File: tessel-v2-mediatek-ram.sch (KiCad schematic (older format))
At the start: 21 parts, among them U201 MT7620N, U501 W9751G6KB-25

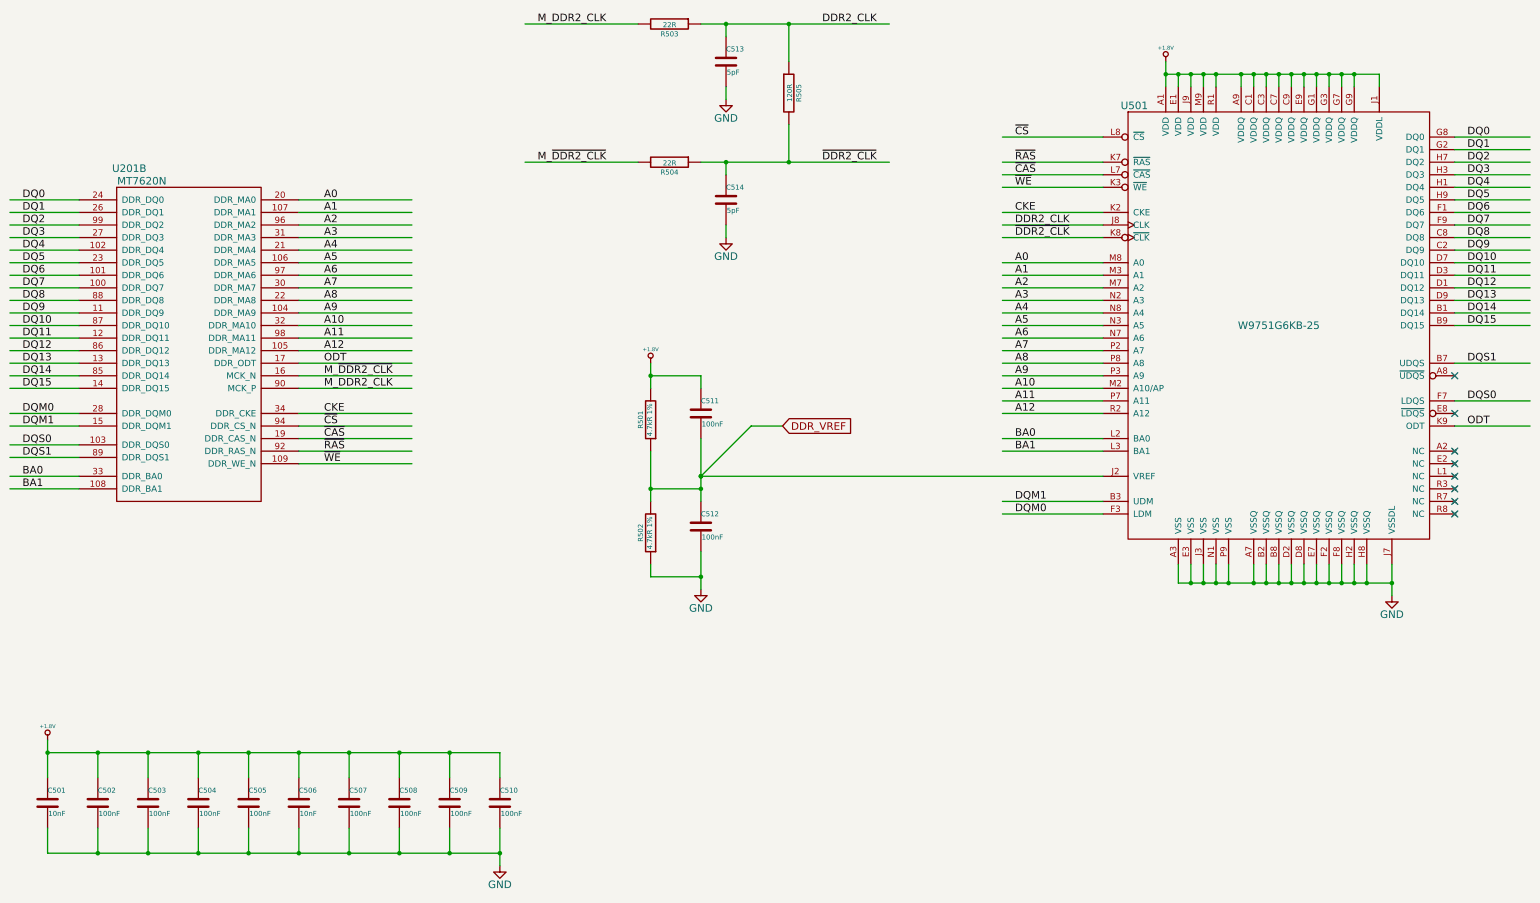
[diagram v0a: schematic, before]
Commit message: annotation did not take?
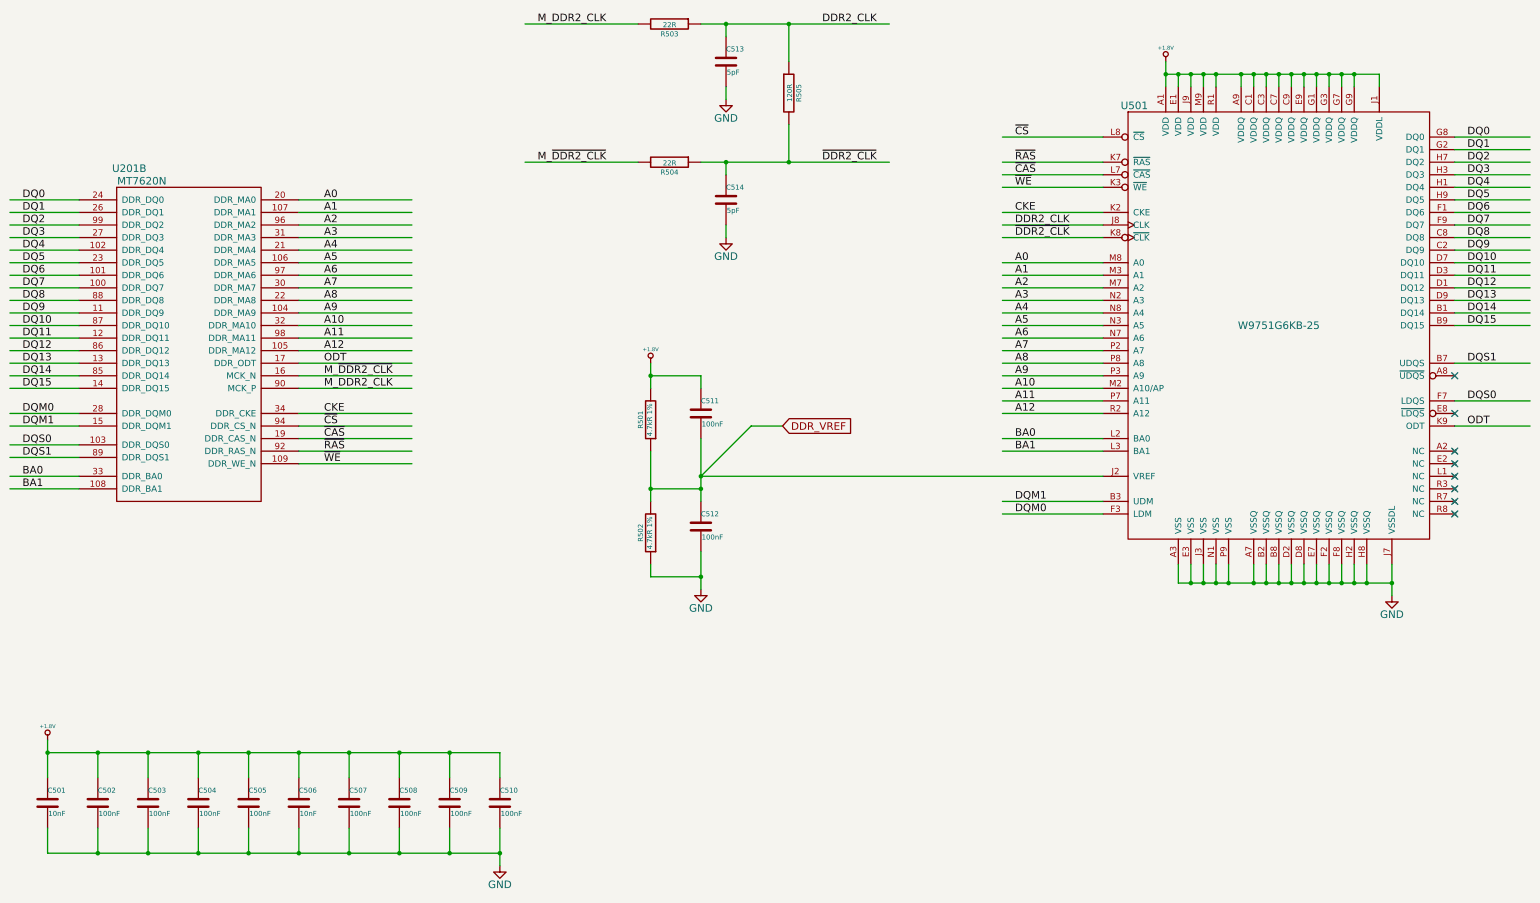
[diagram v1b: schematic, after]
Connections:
- wire segments 222 -> 164
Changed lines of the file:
@@
 	11500 7000 11500 7150
 Wire Wire Line
-	11500 7150 11600 7150
-Wire Wire Line
-	11600 7150 11700 7150
-Wire Wire Line
-	11700 7150 11800 7150
-Wire Wire Line
-	11800 7150 11900 7150
-Wire Wire Line
-	11900 7150 12100 7150
-Wire Wire Line
-	12100 7150 12200 7150
-Wire Wire Line
-	12200 7150 12300 7150
-Wire Wire Line
-	12300 7150 12400 7150
-Wire Wire Line
-	12400 7150 12500 7150
-Wire Wire Line
-	12500 7150 12600 7150
-Wire Wire Line
-	12600 7150 12700 7150
-Wire Wire Line
-	12700 7150 12800 7150
-Wire Wire Line
-	12800 7150 12900 7150
-Wire Wire Line
-	12900 7150 13000 7150
-Wire Wire Line
-	13000 7150 13200 7150
+	11500 7150 13200 7150
 Wire Wire Line
 	11600 7150 11600 7000
@@
 Connection ~ 12200 7150
 Wire Wire Line
-	13200 7000 13200 7150
-Wire Wire Line
-	13200 7150 13200 7250
+	13200 7000 13200 7250
 Wire Wire Line
 	12400 7150 12400 7000
@@
 	4500 5600 5400 5600
 Wire Wire Line
-	7700 2700 7900 2700
-Wire Wire Line
-	7900 2700 8400 2700
-Wire Wire Line
-	8400 2700 9200 2700
+	7700 2700 9200 2700
 Wire Wire Line
 	7900 2800 7900 2700
@@
 	6300 3800 7200 3800
 Wire Wire Line
-	11400 3100 11500 3100
-Wire Wire Line
-	11500 3100 11600 3100
-Wire Wire Line
-	11600 3100 11700 3100
-Wire Wire Line
-	11700 3100 11800 3100
-Wire Wire Line
-	11800 3100 12000 3100
-Wire Wire Line
-	12000 3100 12100 3100
-Wire Wire Line
-	12100 3100 12200 3100
-Wire Wire Line
-	12200 3100 12300 3100
-Wire Wire Line
-	12300 3100 12400 3100
-Wire Wire Line
-	12400 3100 12500 3100
-Wire Wire Line
-	12500 3100 12600 3100
-Wire Wire Line
-	12600 3100 12700 3100
-Wire Wire Line
-	12700 3100 12800 3100
-Wire Wire Line
-	12800 3100 12900 3100
-Wire Wire Line
-	12900 3100 13100 3100
-Wire Wire Line
-	11400 3000 11400 3100
-Wire Wire Line
-	11400 3100 11400 3200
+	11400 3100 13100 3100
+Wire Wire Line
+	11400 3000 11400 3200
 Wire Wire Line
 	11500 3200 11500 3100
@@
 Connection ~ 12900 3100
 Wire Wire Line
-	2500 8400 2500 8500
-Wire Wire Line
-	2500 8500 2500 8700
-Wire Wire Line
-	2500 8500 2900 8500
-Wire Wire Line
-	2900 8500 3300 8500
-Wire Wire Line
-	3300 8500 3700 8500
-Wire Wire Line
-	3700 8500 4100 8500
-Wire Wire Line
-	4100 8500 4500 8500
-Wire Wire Line
-	4500 8500 4900 8500
-Wire Wire Line
-	4900 8500 5300 8500
-Wire Wire Line
-	5300 8500 5700 8500
-Wire Wire Line
-	5700 8500 6100 8500
+	2500 8400 2500 8700
+Wire Wire Line
+	2500 8500 6100 8500
 Wire Wire Line
 	2900 8500 2900 8700
@@
 	4100 9300 4100 9100
 Wire Wire Line
-	2500 9300 2900 9300
-Wire Wire Line
-	2900 9300 3300 9300
-Wire Wire Line
-	3300 9300 3700 9300
-Wire Wire Line
-	3700 9300 4100 9300
-Wire Wire Line
-	4100 9300 4500 9300
-Wire Wire Line
-	4500 9300 4900 9300
-Wire Wire Line
-	4900 9300 5300 9300
-Wire Wire Line
-	5300 9300 5700 9300
-Wire Wire Line
-	5700 9300 6100 9300
+	2500 9300 6100 9300
 Wire Wire Line
 	3700 9300 3700 9100
@@
 Connection ~ 5700 8500
 Wire Wire Line
-	6100 9100 6100 9300
-Wire Wire Line
-	6100 9300 6100 9400
+	6100 9100 6100 9400
 Wire Wire Line
 	5700 9300 5700 9100
@@
 Connection ~ 4900 9300
 Wire Wire Line
-	7300 5400 7300 5500
-Wire Wire Line
-	7300 5500 7300 5600
+	7300 5400 7300 5600
 Wire Wire Line
 	7700 5500 7700 5600
 Wire Wire Line
-	7700 6000 7700 6300
-Wire Wire Line
-	7700 6300 7700 6400
-Wire Wire Line
-	7700 6400 7700 6500
-Wire Wire Line
-	7300 6100 7300 6400
-Wire Wire Line
-	7300 6400 7300 6500
+	7700 6000 7700 6500
+Wire Wire Line
+	7300 6100 7300 6500
 Wire Wire Line
 	7300 6400 7700 6400
@@
 Connection ~ 13200 7150
 Wire Wire Line
-	7700 6900 7700 7100
-Wire Wire Line
-	7700 7100 7700 7200
+	7700 6900 7700 7200
 Wire Wire Line
 	7300 7100 7700 7100
@@
 	10900 4400 10100 4400
 Wire Wire Line
-	7700 3800 7900 3800
-Wire Wire Line
-	7900 3800 8400 3800
-Wire Wire Line
-	8400 3800 9200 3800
+	7700 3800 9200 3800
 Wire Wire Line
 	7900 3800 7900 3900
@@
 Connection ~ 4100 8500
 Wire Wire Line
-	10900 6300 7700 6300
-Wire Wire Line
-	7700 6300 7700 6300
+	7700 6300 10900 6300
 Wire Wire Line
 	8350 5900 8100 5900
 Wire Wire Line
 	8100 5900 7700 6300
-Connection ~ 7700 6300
 $Comp
 L MT7620N U?
